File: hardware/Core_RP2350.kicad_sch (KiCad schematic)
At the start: 70 parts, among them U1 RP2350B-QFN80, U2 LM4040A30IDBZR, U3 W25Q128JVS, U4 W25Q128JVS, U5 W25Q128JVS

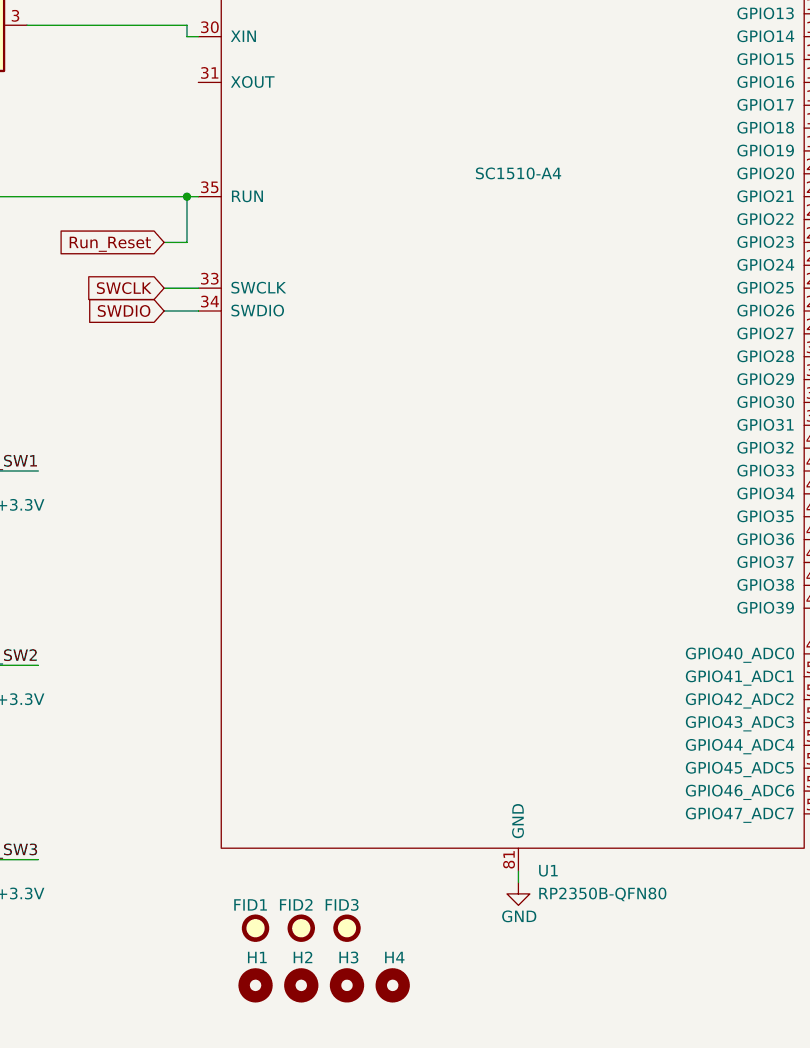
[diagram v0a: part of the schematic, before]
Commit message: BOM cont.
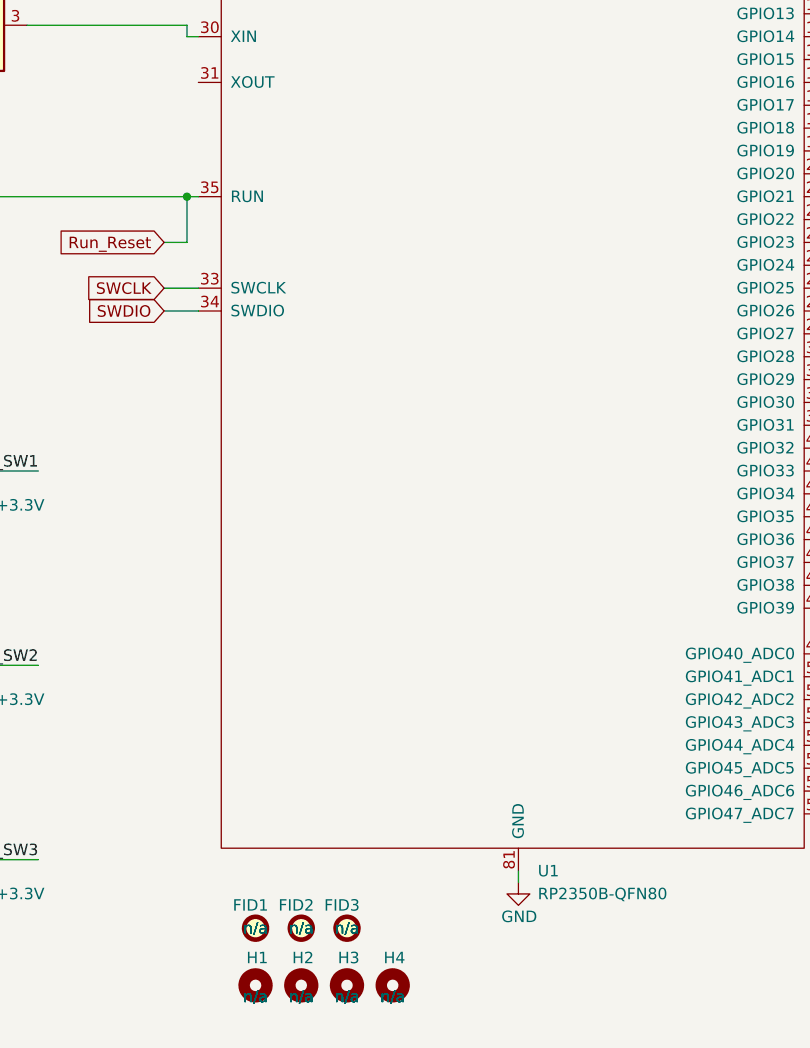
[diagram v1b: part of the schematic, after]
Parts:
- FID1, FID2, FID3: MPN (none) -> n/a; Manufacturer_Name (none) -> n/a; Manufacturer_Part_Number (none) -> n/a
- H1, H2, H3, H4: Link (none) -> n/a; MPN (none) -> n/a; Manufacturer (none) -> n/a; Manufacturer_Name (none) -> n/a; Manufacturer_Part_Number (none) -> n/a
- Jump1: Link (none) -> https://www.digikey.com/en/products/detail/harwin-inc/M20-9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; MPN (none) -> M20-9990246; Manufacturer (none) -> Harwin Inc.; Manufacturer_Name (none) -> Harwin Inc.; Manufacturer_Part_Number (none) -> M20-9990246
